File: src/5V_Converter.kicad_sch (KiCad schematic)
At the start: 16 parts, among them U3 TPS566238RQFR (12V to 5V)

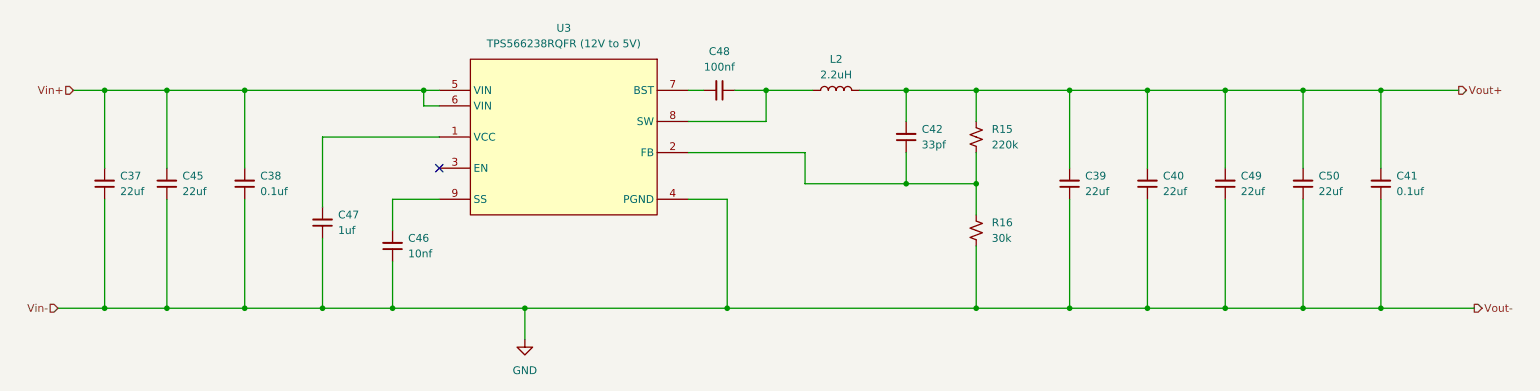
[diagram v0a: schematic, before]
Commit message: Finalized schematic
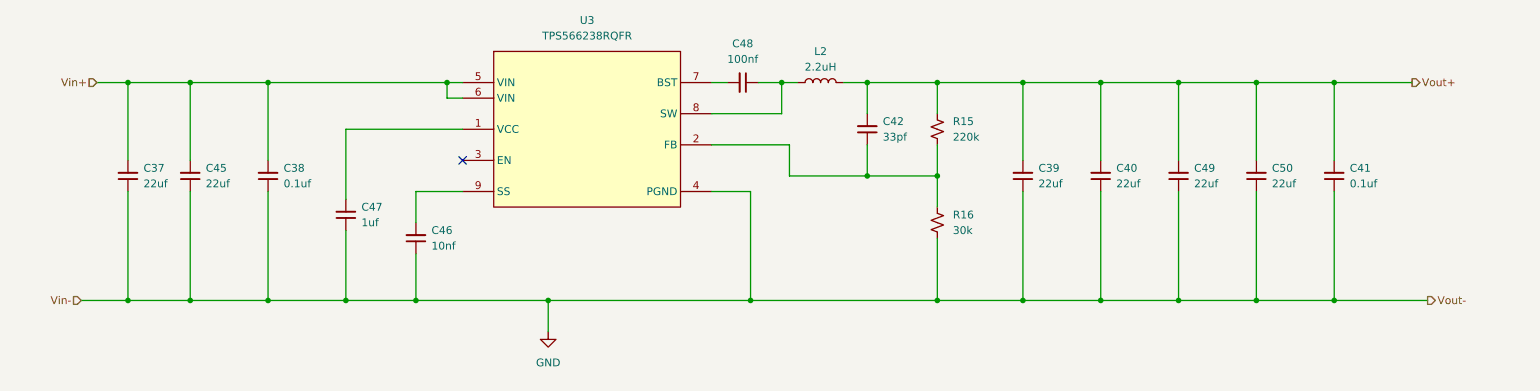
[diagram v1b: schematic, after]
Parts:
- U3: value TPS566238RQFR (12V to 5V) -> TPS566238RQFR
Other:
- moved on the sheet: C37, C38, C39, C40, C41, C42, C45, C46, C47, C48, C49, C50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
